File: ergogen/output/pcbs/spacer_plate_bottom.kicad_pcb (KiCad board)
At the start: 2 copper layers, 71.2 x 109.2 mm, 0 parts

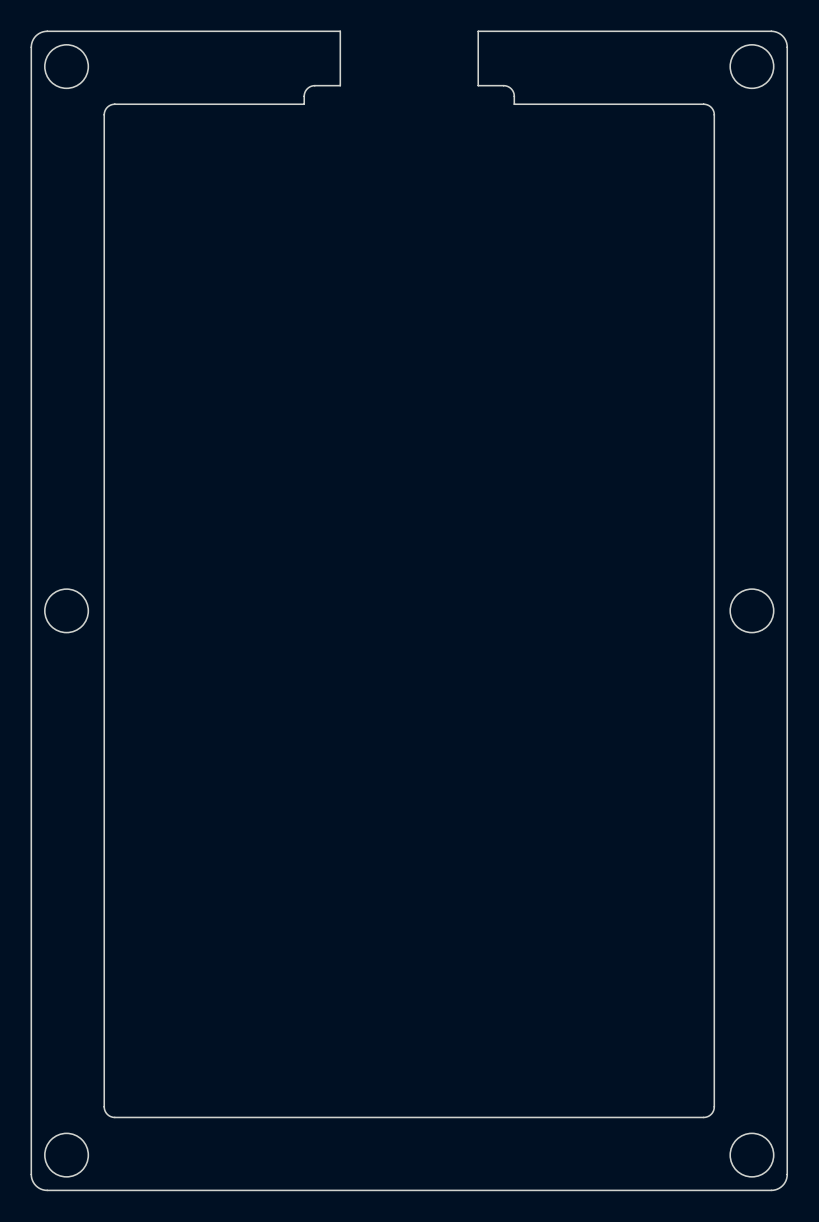
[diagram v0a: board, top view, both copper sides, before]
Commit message: Update assets
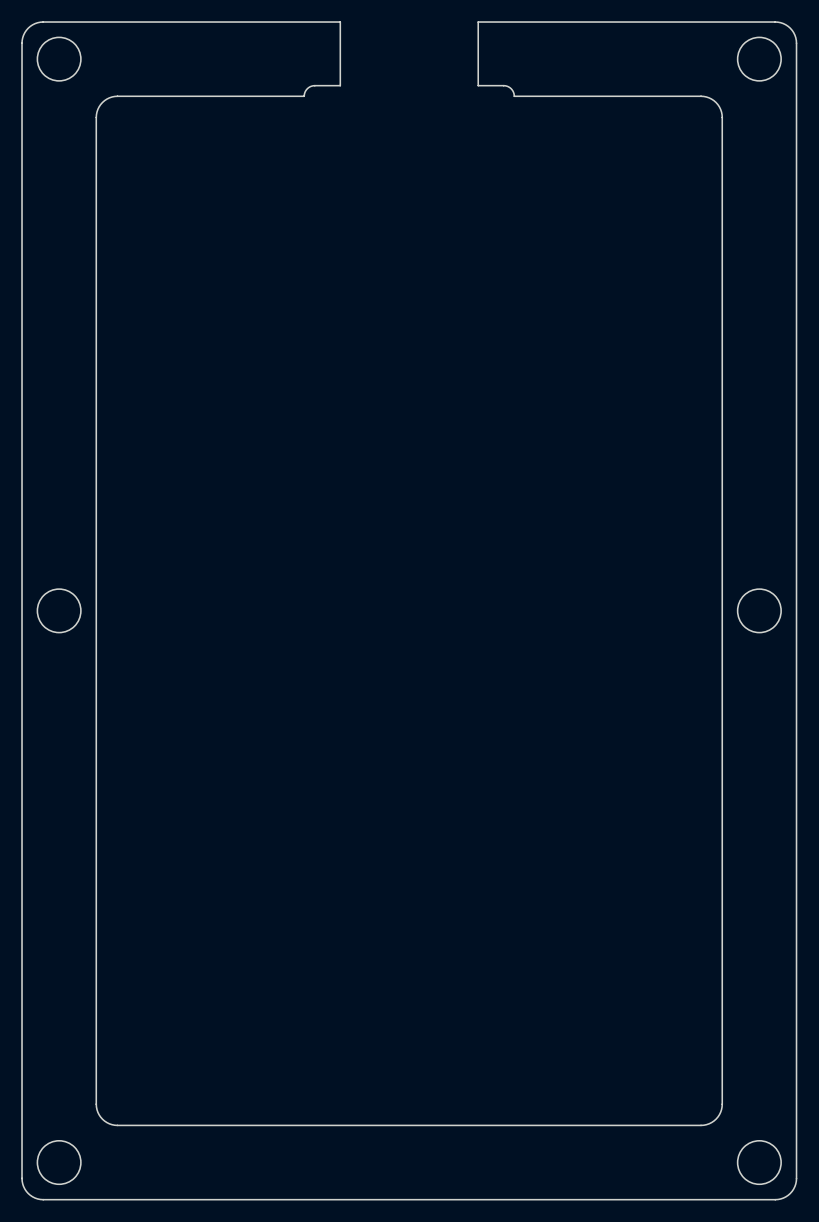
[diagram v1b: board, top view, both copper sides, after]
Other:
- board size 71.2 x 109.2 mm -> 73 x 111 mm
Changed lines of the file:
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@@
     (add_net "")
   )
-            (gr_line (start 44.875 141.625) (end 113.125 141.625) (angle 90) (layer Edge.Cuts) (width 0.15))
-(gr_line (start 114.625 140.125) (end 114.625 33.875) (angle 90) (layer Edge.Cuts) (width 0.15))
-(gr_line (start 113.125 32.375) (end 85.5 32.375) (angle 90) (layer Edge.Cuts) (width 0.15))
-(gr_line (start 72.5 32.375) (end 44.875 32.375) (angle 90) (layer Edge.Cuts) (width 0.15))
-(gr_line (start 43.375 33.875) (end 43.375 140.125) (angle 90) (layer Edge.Cuts) (width 0.15))
-(gr_arc (start 113.125 140.125) (end 113.125 141.625) (angle -90) (layer Edge.Cuts) (width 0.15))
-(gr_arc (start 113.125 33.875) (end 114.625 33.875) (angle -90) (layer Edge.Cuts) (width 0.15))
-(gr_arc (start 44.875 33.875) (end 44.875 32.375) (angle -90) (layer Edge.Cuts) (width 0.15))
-(gr_arc (start 44.875 140.125) (end 43.375 140.125) (angle -90) (layer Edge.Cuts) (width 0.15))
-(gr_line (start 51.25 134.75) (end 106.75 134.75) (angle 90) (layer Edge.Cuts) (width 0.15))
-(gr_line (start 107.75 133.75) (end 107.75 40.25) (angle 90) (layer Edge.Cuts) (width 0.15))
-(gr_line (start 106.75 39.25) (end 88.89999999999999 39.25) (angle 90) (layer Edge.Cuts) (width 0.15))
-(gr_line (start 69.1 39.25) (end 51.25 39.25) (angle 90) (layer Edge.Cuts) (width 0.15))
-(gr_line (start 50.25 40.25) (end 50.25 133.75) (angle 90) (layer Edge.Cuts) (width 0.15))
-(gr_arc (start 106.75 133.75) (end 106.75 134.75) (angle -90) (layer Edge.Cuts) (width 0.15))
-(gr_arc (start 106.75 40.25) (end 107.75 40.25) (angle -90) (layer Edge.Cuts) (width 0.15))
-(gr_arc (start 51.25 40.25) (end 51.25 39.25) (angle -90) (layer Edge.Cuts) (width 0.15))
-(gr_arc (start 51.25 133.75) (end 50.25 133.75) (angle -90) (layer Edge.Cuts) (width 0.15))
-(gr_circle (center 46.7 35.7) (end 48.75 35.7) (layer Edge.Cuts) (width 0.15))
-(gr_circle (center 111.3 35.7) (end 113.35 35.7) (layer Edge.Cuts) (width 0.15))
-(gr_circle (center 46.7 87) (end 48.75 87) (layer Edge.Cuts) (width 0.15))
-(gr_circle (center 111.3 87) (end 113.35 87) (layer Edge.Cuts) (width 0.15))
-(gr_circle (center 46.7 138.3) (end 48.75 138.3) (layer Edge.Cuts) (width 0.15))
-(gr_circle (center 111.3 138.3) (end 113.35 138.3) (layer Edge.Cuts) (width 0.15))
-(gr_line (start 88.89999999999999 39.25) (end 88.89999999999999 38.5) (angle 90) (layer Edge.Cuts) (width 0.15))
+            (gr_line (start 44.5 142.5) (end 113.5 142.5) (angle 90) (layer Edge.Cuts) (width 0.15))
+(gr_line (start 115.5 140.5) (end 115.5 33.5) (angle 90) (layer Edge.Cuts) (width 0.15))
+(gr_line (start 44.5 31.5) (end 72.5 31.5) (angle 90) (layer Edge.Cuts) (width 0.15))
+(gr_line (start 85.5 31.5) (end 113.5 31.5) (angle 90) (layer Edge.Cuts) (width 0.15))
+(gr_line (start 42.5 140.5) (end 42.5 33.5) (angle 90) (layer Edge.Cuts) (width 0.15))
+(gr_arc (start 113.5 140.5) (end 113.5 142.5) (angle -90) (layer Edge.Cuts) (width 0.15))
+(gr_arc (start 113.5 33.5) (end 115.5 33.5) (angle -90) (layer Edge.Cuts) (width 0.15))
+(gr_arc (start 44.5 33.5) (end 44.5 31.5) (angle -90) (layer Edge.Cuts) (width 0.15))
+(gr_arc (start 44.5 140.5) (end 42.5 140.5) (angle -90) (layer Edge.Cuts) (width 0.15))
+(gr_line (start 51.5 135.5) (end 106.5 135.5) (angle 90) (layer Edge.Cuts) (width 0.15))
+(gr_arc (start 106.5 133.5) (end 106.5 135.5) (angle -90) (layer Edge.Cuts) (width 0.15))
+(gr_line (start 108.5 133.5) (end 108.5 40.5) (angle 90) (layer Edge.Cuts) (width 0.15))
+(gr_arc (start 106.5 40.5) (end 108.5 40.5) (angle -90) (layer Edge.Cuts) (width 0.15))
+(gr_line (start 106.5 38.5) (end 88.89999999999999 38.5) (angle 90) (layer Edge.Cuts) (width 0.15))
+(gr_line (start 69.1 38.5) (end 51.5 38.5) (angle 90) (layer Edge.Cuts) (width 0.15))
+(gr_arc (start 51.5 40.5) (end 51.5 38.5) (angle -90) (layer Edge.Cuts) (width 0.15))
+(gr_line (start 49.5 40.5) (end 49.5 133.5) (angle 90) (layer Edge.Cuts) (width 0.15))
+(gr_arc (start 51.5 133.5) (end 49.5 133.5) (angle -90) (layer Edge.Cuts) (width 0.15))
+(gr_circle (center 46 35) (end 48.05 35) (layer Edge.Cuts) (width 0.15))
+(gr_circle (center 112 35) (end 114.05 35) (layer Edge.Cuts) (width 0.15))
+(gr_circle (center 46 87) (end 48.05 87) (layer Edge.Cuts) (width 0.15))
+(gr_circle (center 112 87) (end 114.05 87) (layer Edge.Cuts) (width 0.15))
+(gr_circle (center 46 139) (end 48.05 139) (layer Edge.Cuts) (width 0.15))
+(gr_circle (center 112 139) (end 114.05 139) (layer Edge.Cuts) (width 0.15))
 (gr_arc (start 87.89999999999999 38.5) (end 88.89999999999999 38.5) (angle -90) (layer Edge.Cuts) (width 0.15))
 (gr_line (start 87.89999999999999 37.5) (end 85.5 37.5) (angle 90) (layer Edge.Cuts) (width 0.15))
 (gr_line (start 72.5 37.5) (end 70.1 37.5) (angle 90) (layer Edge.Cuts) (width 0.15))
 (gr_arc (start 70.1 38.5) (end 70.1 37.5) (angle -90) (layer Edge.Cuts) (width 0.15))
-(gr_line (start 69.1 38.5) (end 69.1 39.25) (angle 90) (layer Edge.Cuts) (width 0.15))
-(gr_line (start 85.5 37.5) (end 85.5 32.375) (angle 90) (layer Edge.Cuts) (width 0.15))
-(gr_line (start 72.5 32.375) (end 72.5 37.5) (angle 90) (layer Edge.Cuts) (width 0.15))
+(gr_line (start 85.5 37.5) (end 85.5 31.5) (angle 90) (layer Edge.Cuts) (width 0.15))
+(gr_line (start 72.5 31.5) (end 72.5 37.5) (angle 90) (layer Edge.Cuts) (width 0.15))
 )
